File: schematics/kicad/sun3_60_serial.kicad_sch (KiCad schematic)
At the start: 13 parts, among them J1 KB/Mouse, J2 Serial A/B, J3 Mini-DIN-8, J6 DB25_Socket, J7 DB25_Socket, U400 Z8530, U401 Z8530, U402 4.9152 Mhz, U404 74ALS04, U408 74ALS04, X52 100nF 0402

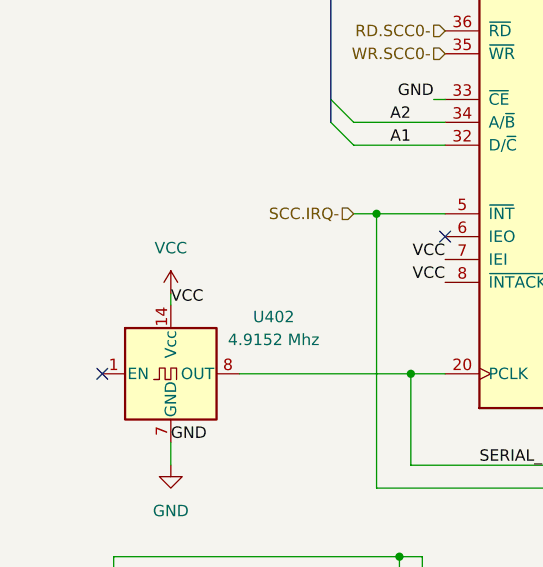
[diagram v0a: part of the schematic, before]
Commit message: ongoing
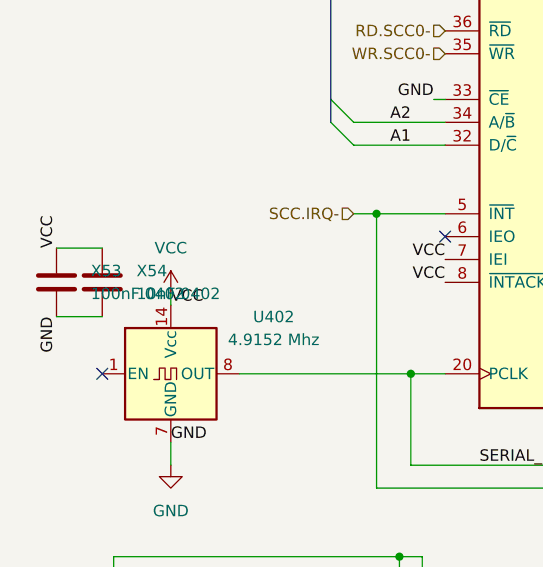
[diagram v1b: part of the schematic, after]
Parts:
- added X53: 100nF 0402, Capacitor_SMD:C_0402_1005Metric, symbol Device:C
- added X54: 10nF 0402, Capacitor_SMD:C_0402_1005Metric, symbol Device:C
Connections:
- net GND: now also X53.2, X54.2
- net VCC: now also X53.1, X54.1
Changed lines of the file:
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@@
+	(wire
+		(pts
+			(xy 16.51 88.9) (xy 21.59 88.9)
+		)
+		(stroke
+			(width 0)
+			(type default)
+		)
+	)
 	(wire
 		(pts
@@
 		(pts
 			(xy 144.78 154.94) (xy 148.59 154.94)
+		)
+		(stroke
+			(width 0)
+			(type default)
+		)
+	)
+	(wire
+		(pts
+			(xy 16.51 96.52) (xy 21.59 96.52)
 		)
 		(stroke
@@
 		)
 	)
+	(label "VCC"
+		(at 16.51 88.9 90)
+		(effects
+			(font
+				(size 1.27 1.27)
+			)
+			(justify left bottom)
+		)
+	)
 	(label "A2"
 		(at 55.88 74.93 180)
@@
 			)
 			(justify left bottom)
+		)
+	)
+	(label "GND"
+		(at 16.51 96.52 270)
+		(effects
+			(font
+				(size 1.27 1.27)
+			)
+			(justify right bottom)
 		)
 	)
@@
 	)
 	(symbol
+		(lib_id "Device:C")
+		(at 21.59 92.71 0)
+		(unit 1)
+		(exclude_from_sim no)
+		(in_bom yes)
+		(on_board yes)
+		(dnp no)
+		(fields_autoplaced yes)
+		(property "Reference" "X54"
+			(at 25.4 91.4399 0)
+			(effects
+				(font
+					(size 1.27 1.27)
+				)
+				(justify left)
+			)
+		)
+		(property "Value" "10nF 0402"
+			(at 25.4 93.9799 0)
+			(effects
+				(font
+					(size 1.27 1.27)
+				)
+				(justify left)
+			)
+		)
+		(property "Footprint" "Capacitor_SMD:C_0402_1005Metric"
+			(at 22.5552 96.52 0)
+			(effects
+				(font
+					(size 1.27 1.27)
+				)
+				(hide yes)
+			)
+		)
+		(property "Datasheet" "~"
+			(at 21.59 92.71 0)
+			(effects
+				(font
+					(size 1.27 1.27)
+				)
+				(hide yes)
+			)
+		)
+		(property "Description" "Unpolarized capacitor"
+			(at 21.59 92.71 0)
+			(effects
+				(font
+					(size 1.27 1.27)
+				)
+				(hide yes)
+			)
+		)
+		(property "MPN" "CL05B103KB5NNNC"
+			(at 21.59 92.71 0)
+			(effects
+				(font
+					(size 1.27 1.27)
+				)
+				(hide yes)
+			)
+		)
+		(pin "1"
+		)
+		(pin "2"
+		)
+		(instances
+			(project "sun3_60"
+				(path "/d6b5cf90-8df0-4384-868a-524abed7c432/054c9f34-4c69-4214-aead-9eddc8182f56"
+					(reference "X54")
+					(unit 1)
+				)
+			)
+		)
+	)
+	(symbol
 		(lib_id "Device:R_Pack04_SIP")
 		(at 201.93 129.54 90)
@@
 				)
 			)
+		)
+	)
+	(symbol
+		(lib_id "Device:C")
+		(at 16.51 92.71 0)
+		(unit 1)
+		(exclude_from_sim no)
+		(in_bom yes)
+		(on_board yes)
+		(dnp no)
+		(fields_autoplaced yes)
+		(property "Reference" "X53"
+			(at 20.32 91.4399 0)
+			(effects
+				(font
+					(size 1.27 1.27)
+				)
+				(justify left)
+			)
+		)
+		(property "Value" "100nF 0402"
+			(at 20.32 93.9799 0)
+			(effects
+				(font
+					(size 1.27 1.27)
+				)
+				(justify left)
+			)
+		)
+		(property "Footprint" "Capacitor_SMD:C_0402_1005Metric"
+			(at 17.4752 96.52 0)
+			(effects
+				(font
+					(size 1.27 1.27)
+				)
+				(hide yes)
+			)
+		)
+		(property "Datasheet" "~"
+			(at 16.51 92.71 0)
+			(effects
+				(font
+					(size 1.27 1.27)
+				)
+				(hide yes)
+			)
+		)
+		(property "Description" "Unpolarized capacitor"
+			(at 16.51 92.71 0)
+			(effects
+				(font
+					(size 1.27 1.27)
+				)
+				(hide yes)
+			)
+		)
+		(property "MPN" "CL05B104KO5NNNC"
+			(at 16.51 92.71 0)
+			(effects
+				(font
+					(size 1.27 1.27)
+				)
+				(hide yes)
+			)
+		)
+		(pin "1"
+		)
+		(pin "2"
+		)
+		(instances
+			(project "sun3_60"
+				(path "/d6b5cf90-8df0-4384-868a-524abed7c432/054c9f34-4c69-4214-aead-9eddc8182f56"
+					(reference "X53")
+					(unit 1)
+				)
+			)
